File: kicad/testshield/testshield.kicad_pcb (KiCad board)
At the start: 2 copper layers, 13 parts, among them J1 ISP/PDI, J2 Raspiheader, SW1 Reset, U1 ATMEGA328P-PU

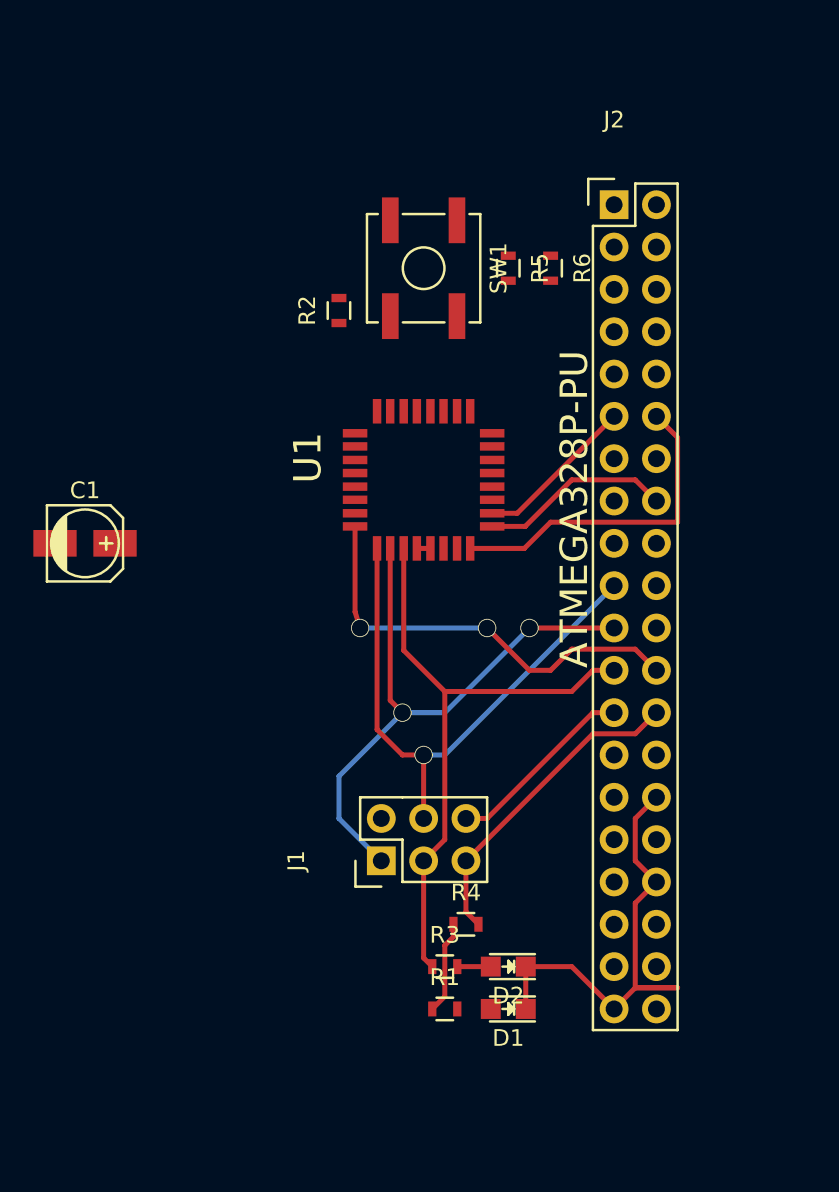
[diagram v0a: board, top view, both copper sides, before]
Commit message: pcb routes WIP
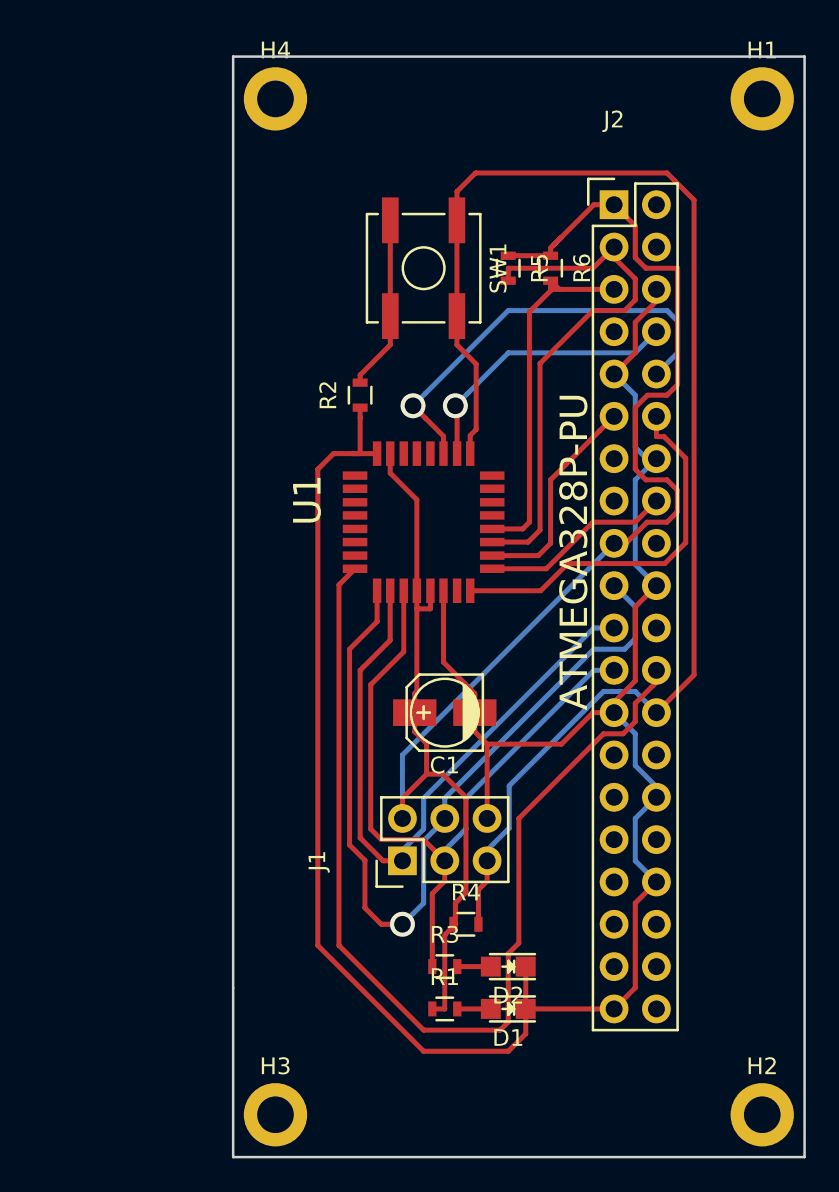
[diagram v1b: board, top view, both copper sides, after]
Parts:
- added H1: MountingHole_2.2mm_M2_ISO14580_Pad, Mounting_Holes:MountingHole_2.2mm_M2_ISO14580_Pad, F.Cu at (175.3, 95.2)
- added H2: MountingHole_2.2mm_M2_ISO14580_Pad, Mounting_Holes:MountingHole_2.2mm_M2_ISO14580_Pad, F.Cu at (175.3, 156.2)
- added H3: MountingHole_2.2mm_M2_ISO14580_Pad, Mounting_Holes:MountingHole_2.2mm_M2_ISO14580_Pad, F.Cu at (146.1, 156.2)
- added H4: MountingHole_2.2mm_M2_ISO14580_Pad, Mounting_Holes:MountingHole_2.2mm_M2_ISO14580_Pad, F.Cu at (146.1, 95.2)
- moved C1 23.9 mm to (156.2, 132.1), turned to 180 degrees
- moved R2 5.24 mm to (151.1, 113.0)
- moved U1 2.54 mm to (154.9, 120.7)
- moved J1 1.27 mm to (153.7, 141.0)
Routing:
- net +3V3: track 6.42 -> 102.0 mm
- net GNDD: track 40.3 -> 135.8 mm
- net /RST: track 19.2 -> 84.2 mm
- net /SS: track 26.0 -> 60.9 mm, vias 2 -> 0
- net /SDA: track 0.00 -> 31.9 mm
- net /RX: track 0.00 -> 25.8 mm, vias 0 -> 1
- net /SCL: track 0.00 -> 22.1 mm
- net /TX: track 0.00 -> 16.8 mm, vias 0 -> 1
- net /MOSI: track 33.7 -> 50.5 mm
- net Net-(R2-Pad2): track 0.00 -> 10.5 mm
- net /SCK: track 37.5 -> 43.4 mm
- net /GPIO17: track 9.72 -> 13.0 mm
- net /PWM: track 20.0 -> 22.7 mm
- net /MISO: track 36.5 -> 38.6 mm, vias 2 -> 0
- net Net-(D1-Pad2): track 0.00 -> 2.01 mm
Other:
- board outline added: 34.3 x 66 mm
- net class Default: via_dia 1.1 -> 1.5
